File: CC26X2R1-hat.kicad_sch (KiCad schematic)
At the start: 6 parts, among them J1 Conn_01x10_Female, J2 Conn_01x10_Female, J3 Conn_01x07, J4 Conn_01x10_Female, J5 Conn_01x10_Female, U1 CC26X2R1

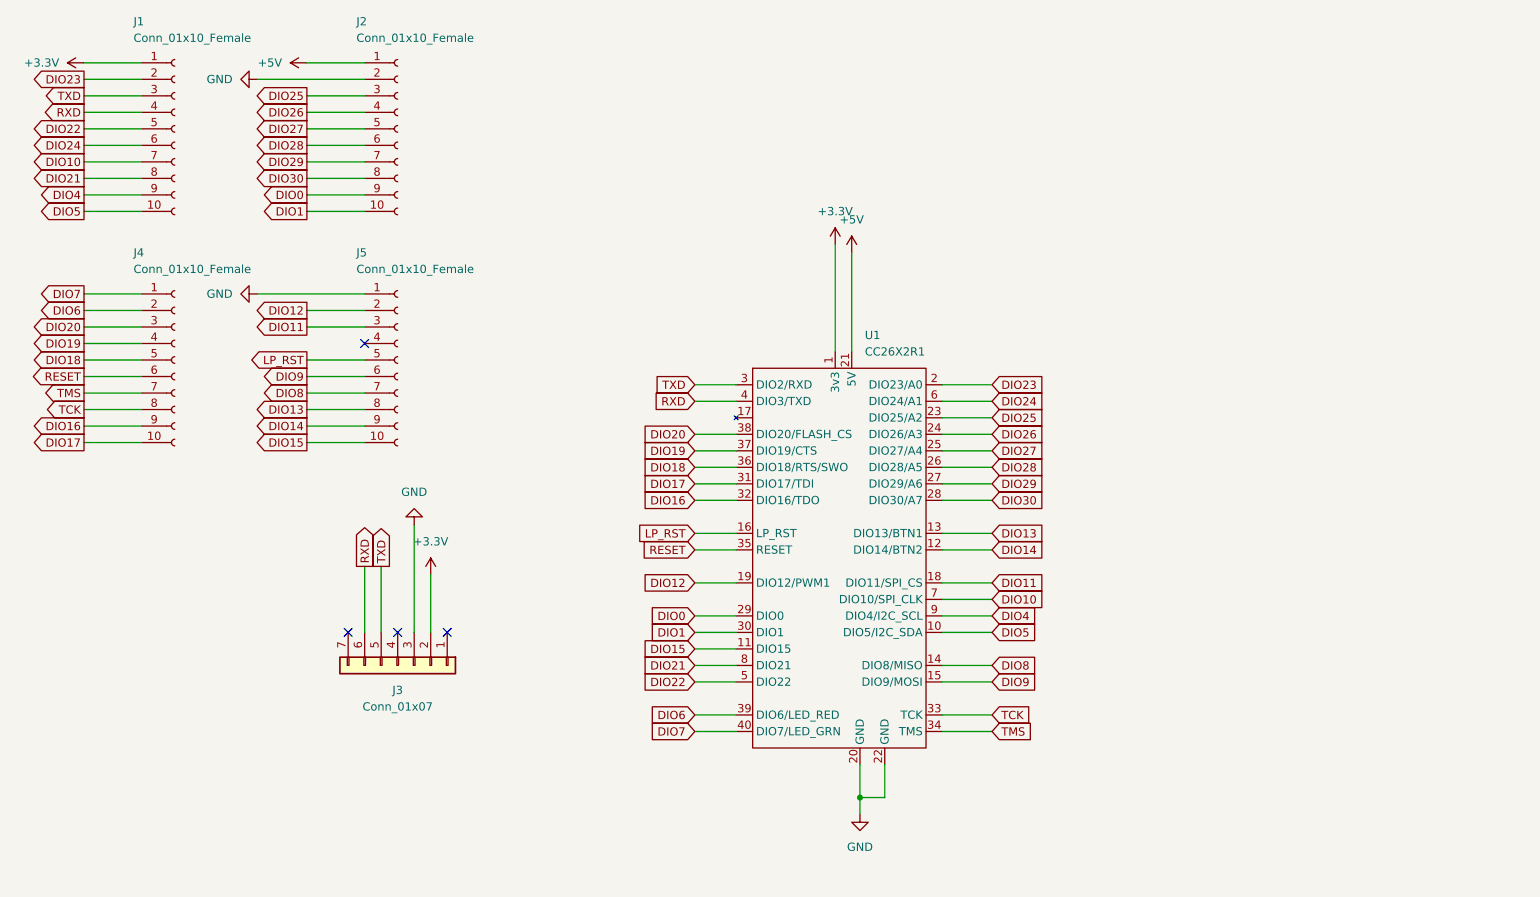
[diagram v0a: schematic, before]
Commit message: v0.1
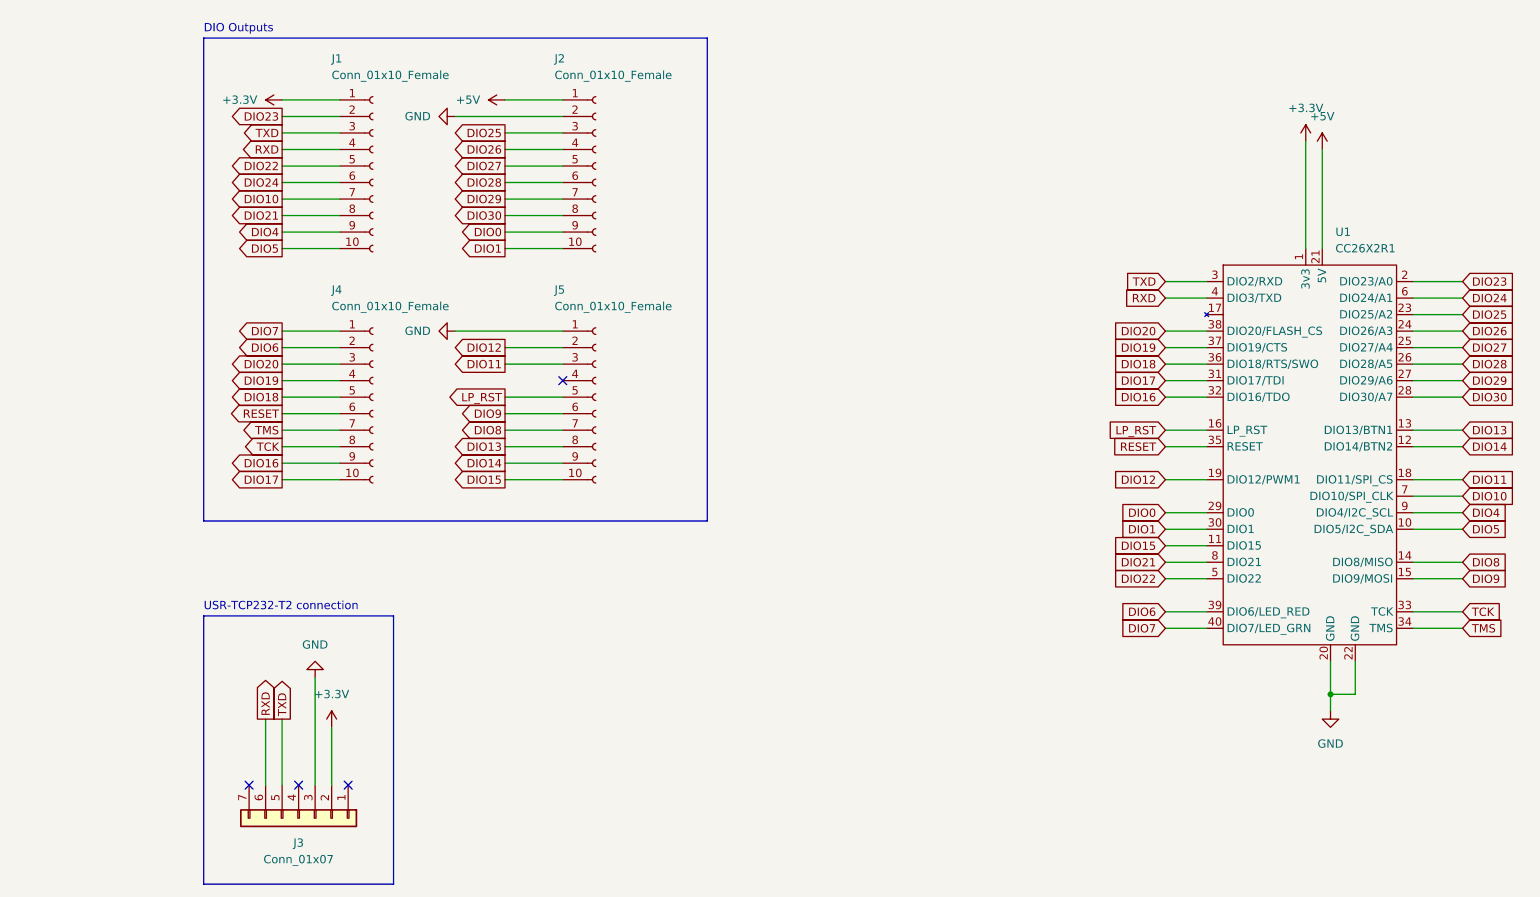
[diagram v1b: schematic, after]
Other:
- note added: "DIO Outputs"
- note added: "USR-TCP232-T2 connection"
- moved on the sheet: J1, J2, J3, J4, J5, U1

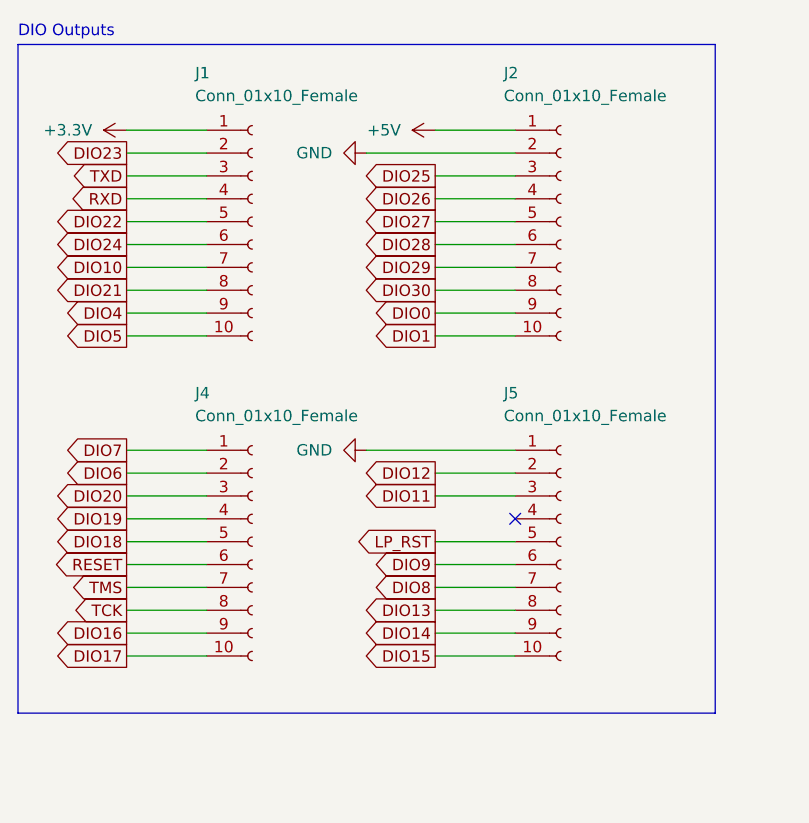
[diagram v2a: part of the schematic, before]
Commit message: v0.3
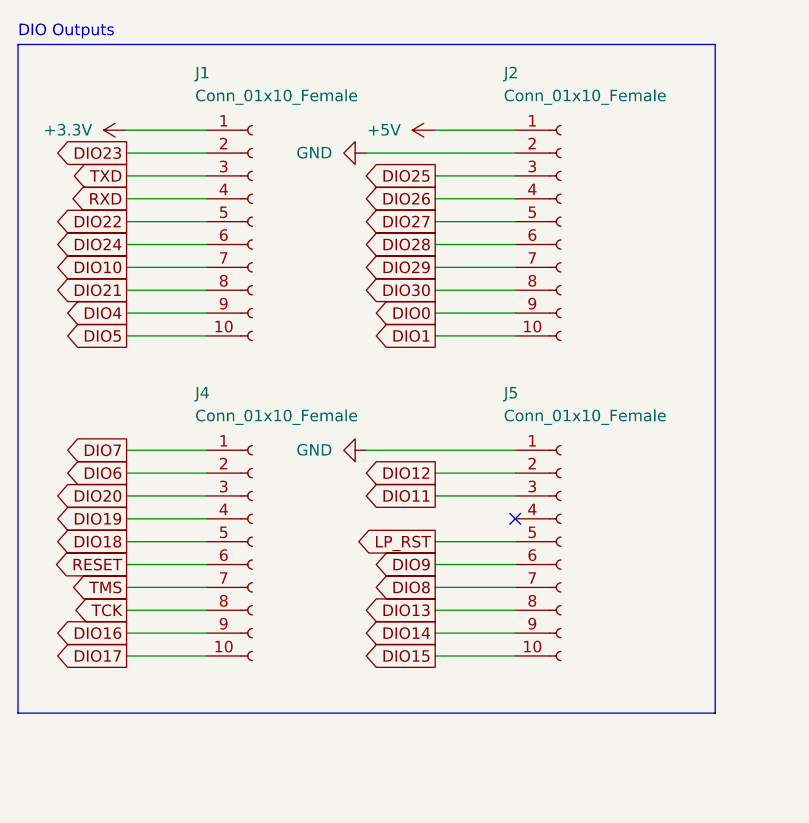
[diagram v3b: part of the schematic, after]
